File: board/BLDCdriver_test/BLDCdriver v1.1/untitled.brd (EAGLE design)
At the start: 46 x 65 mm, 28 parts, among them M1 JST-XH-03-PIN-LONG-PAD, X1 JST-XH-02-PIN-LONG-PAD, X2 JST-XH-06-PIN-ROUND-PAD, X4 JST-XH-04-PIN-ROUND-PAD

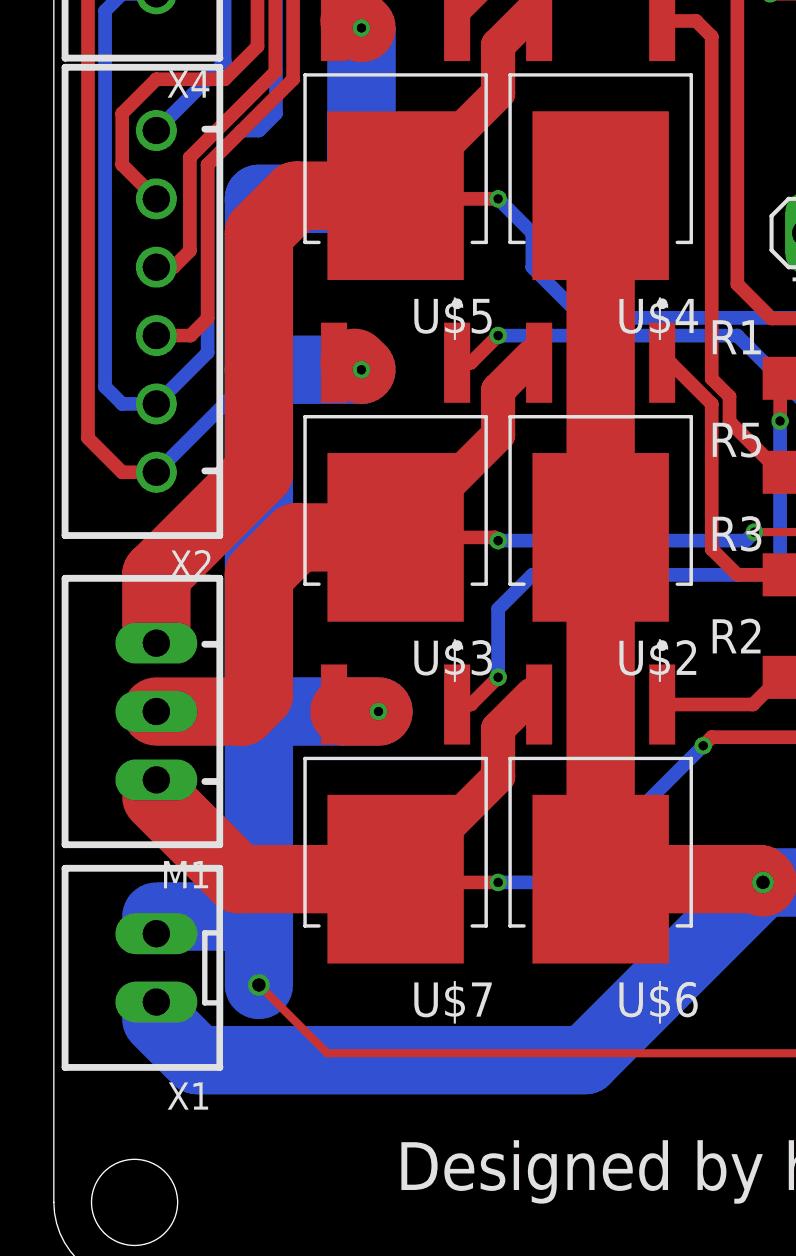
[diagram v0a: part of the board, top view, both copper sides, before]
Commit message: update motordriver
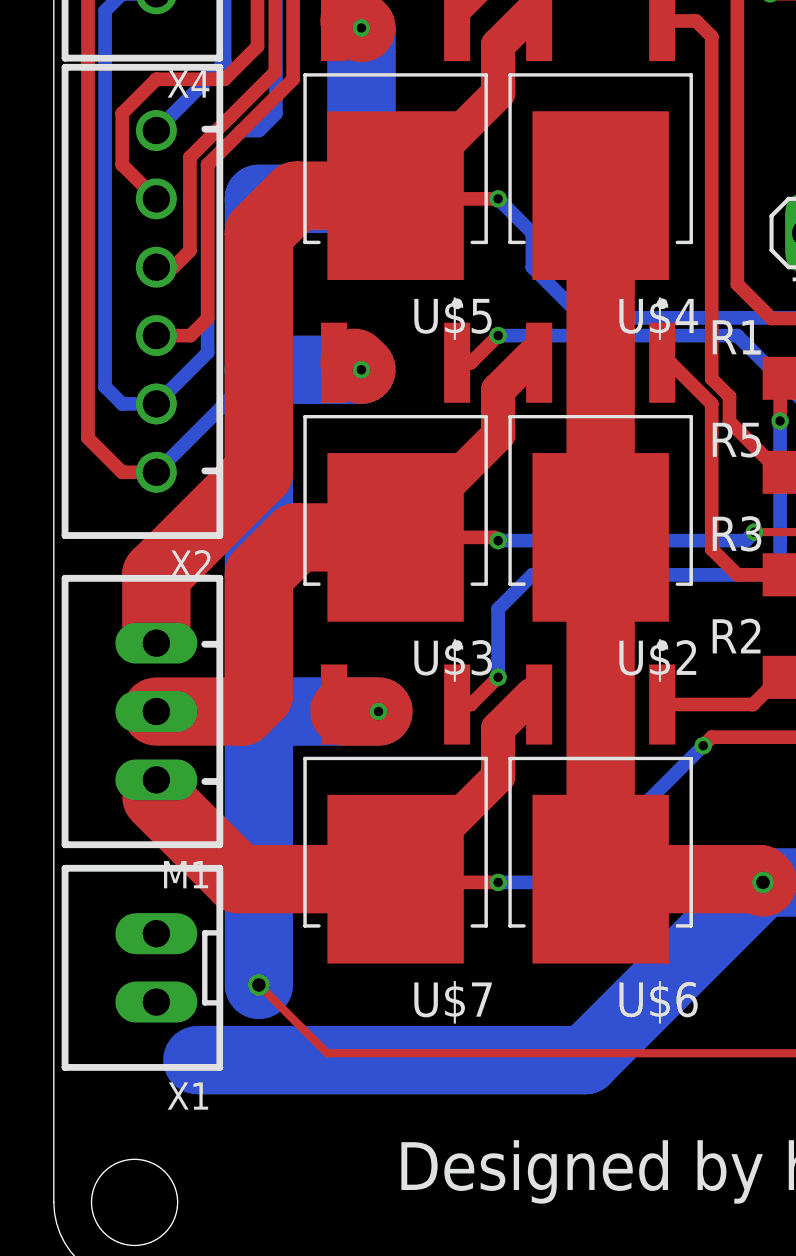
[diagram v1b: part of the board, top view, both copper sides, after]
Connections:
- net GND: now also X1.1; no longer X1.2
- net VCC: now also X1.2; no longer X1.1
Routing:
- net GND: track 201.4 -> 196.9 mm
- net VCC: track 89.3 -> 86.5 mm
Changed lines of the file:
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@@
 <contactref element="U$5" pad="3"/>
 <contactref element="U$1" pad="8"/>
-<contactref element="X1" pad="2"/>
 <via x="7.62" y="5.08" extent="1-16" drill="0.5"/>
-<wire x1="7.62" y1="5.08" x2="7.62" y2="7.62" width="2.54" layer="16"/>
-<wire x1="7.62" y1="7.62" x2="7.62" y2="15.24" width="2.54" layer="16"/>
+<wire x1="7.62" y1="5.08" x2="7.62" y2="15.24" width="2.54" layer="16"/>
 <wire x1="7.62" y1="15.24" x2="7.62" y2="27.94" width="2.54" layer="16"/>
 <contactref element="SV1" pad="2"/>
@@
 <wire x1="10.795" y1="34.29" x2="7.62" y2="34.29" width="2.54" layer="16"/>
 <wire x1="11.43" y1="40.64" x2="11.17" y2="40.9" width="2.54" layer="1"/>
-<wire x1="3.81" y1="6.985" x2="3.81" y2="7.62" width="0.3048" layer="16"/>
-<wire x1="3.81" y1="7.62" x2="7.62" y2="7.62" width="2.54" layer="16"/>
 <wire x1="10.535" y1="15.5" x2="10.795" y2="15.24" width="0.508" layer="1"/>
 <wire x1="10.795" y1="15.24" x2="12.065" y2="15.24" width="2.54" layer="1"/>
@@
 <wire x1="6.35" y1="39.37" x2="3.81" y2="36.83" width="0.508" layer="16"/>
 <wire x1="6.35" y1="44.45" x2="6.35" y2="39.37" width="0.508" layer="16"/>
+<contactref element="X1" pad="1"/>
+<wire x1="3.81" y1="4.445" x2="7.62" y2="5.08" width="0" layer="19" extent="1-1"/>
 </signal>
 <signal name="N$12">
@@
 <contactref element="D3" pad="A"/>
 <contactref element="U$1" pad="7"/>
-<contactref element="X1" pad="1"/>
 <wire x1="20.32" y1="9.01" x2="20.32" y2="21.71" width="2.54" layer="1"/>
-<wire x1="20.32" y1="22.86" x2="20.32" y2="34.41" width="2.54" layer="1"/>
+<wire x1="20.32" y1="21.71" x2="20.32" y2="34.41" width="2.54" layer="1"/>
 <wire x1="35.045" y1="12.7" x2="35.045" y2="8.89" width="1.27" layer="1"/>
 <wire x1="35.045" y1="8.89" x2="35.045" y2="5.08" width="1.27" layer="1"/>
@@
 <wire x1="39.7891" y1="22.225" x2="39.7891" y2="16.2941" width="0.3048" layer="1"/>
 <wire x1="39.7891" y1="16.2941" x2="36.195" y2="12.7" width="0.3048" layer="1"/>
-<wire x1="3.81" y1="4.445" x2="3.81" y2="3.81" width="0.508" layer="16"/>
-<wire x1="3.81" y1="3.81" x2="5.334" y2="2.286" width="2.54" layer="16"/>
 <wire x1="19.7485" y1="2.286" x2="26.3525" y2="8.89" width="2.54" layer="16"/>
 <wire x1="5.334" y1="2.286" x2="19.7485" y2="2.286" width="2.54" layer="16"/>
-<wire x1="20.32" y1="21.71" x2="20.32" y2="22.86" width="2.54" layer="1"/>
+<contactref element="X1" pad="2"/>
+<wire x1="5.334" y1="2.286" x2="3.81" y2="6.985" width="0" layer="19" extent="16-16"/>
 </signal>
 <signal name="N$15">

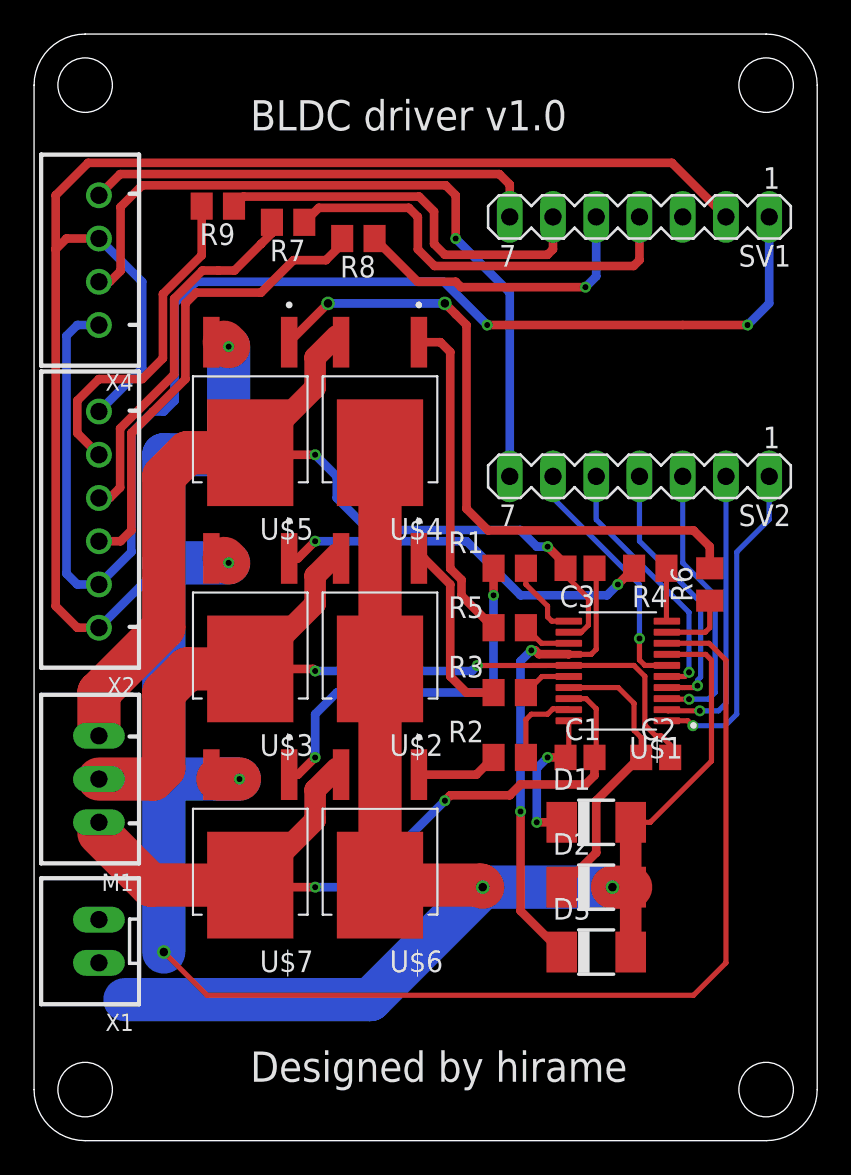
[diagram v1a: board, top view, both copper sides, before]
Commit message: marge前のファイル
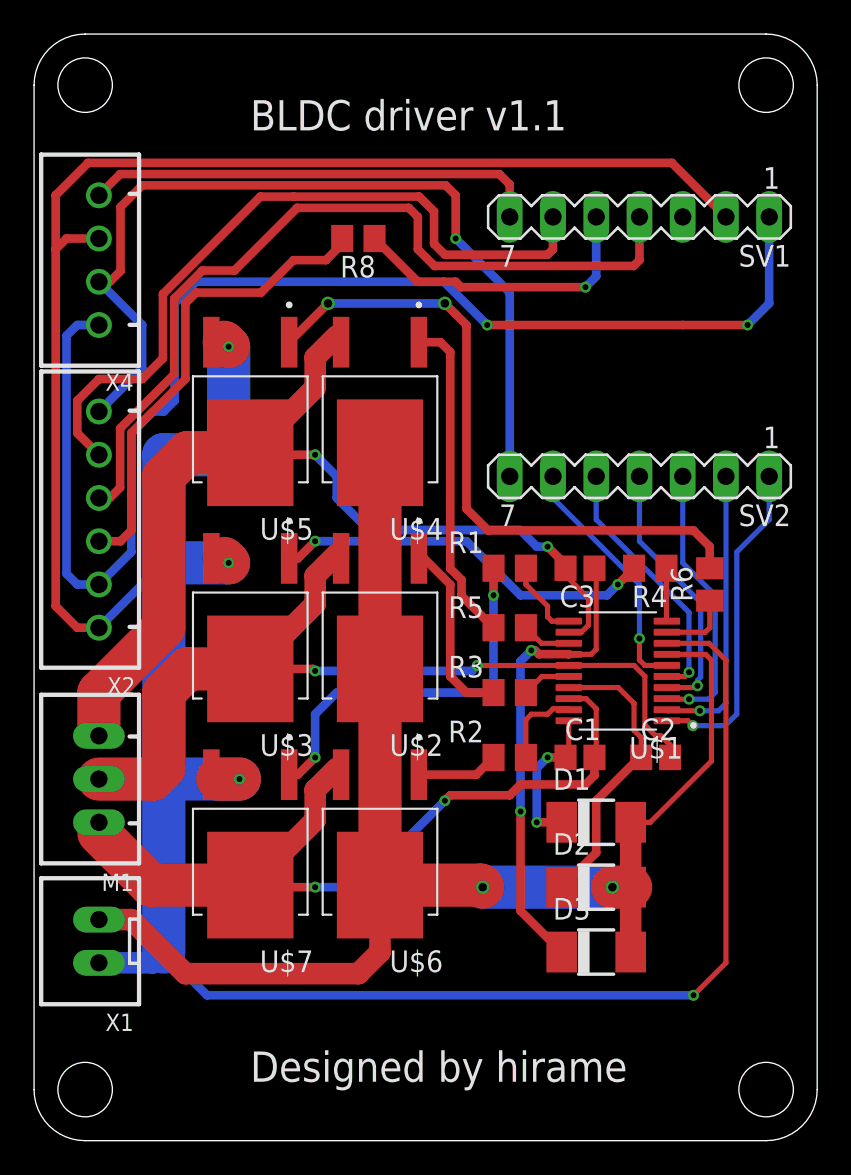
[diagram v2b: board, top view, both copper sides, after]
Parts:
- removed R7, R9: 300Ω, adafruit:M2012
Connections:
- removed net N$11: R7.1, SV1.4
- removed net N$20: R9.1, SV1.6
- net GND: no longer X2.6
- net MOSI: now also SV1.4; no longer R7.2
- net SCK: now also SV1.6; no longer R9.2
- net TX: now also X2.6
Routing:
- net MOSI: track 21.9 -> 48.7 mm
- net N$11: track 25.3 -> 0.00 mm
- net SCK: track 19.6 -> 43.4 mm
- net N$20: track 23.5 -> 0.00 mm
- net TX: track 43.6 -> 53.3 mm
- net GND: track 196.9 -> 188.7 mm
- net VCC: track 86.5 -> 85.0 mm
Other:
- board text added: "BLDC driver v1.1"
- board text removed: "BLDC driver v1.0"
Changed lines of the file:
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@@
 <?xml version="1.0" encoding="utf-8"?>
 <!DOCTYPE eagle SYSTEM "eagle.dtd">
-<eagle version="9.6.1">
+<eagle version="9.6.2">
 <drawing>
 <settings>
@@
 <wire x1="43" y1="-6" x2="46" y2="-3" width="0.001" layer="20" curve="90"/>
 <text x="12.7" y="-2.54" size="1.778" layer="25" font="vector">Designed by hirame</text>
-<text x="12.7" y="53.34" size="1.778" layer="25" font="vector">BLDC driver v1.0</text>
+<text x="12.7" y="53.34" size="1.778" layer="25" font="vector">BLDC driver v1.1</text>
 </plain>
 <attributes>
@@
 <attribute name="VALUE" x="-0.0825" y="39.7175" size="1.016" layer="27" ratio="10" rot="R90"/>
 </element>
-<element name="R7" library="adafruit" package="M2012" value="300Ω" x="14.9225" y="47.9425" smashed="yes" rot="R180">
-<attribute name="NAME" x="15.9385" y="46.9265" size="1.27" layer="25" rot="R180"/>
-<attribute name="VALUE" x="15.9385" y="50.2285" size="1.27" layer="27" rot="R180"/>
-</element>
 <element name="R8" library="adafruit" package="M2012" value="300Ω" x="19.05" y="46.99" smashed="yes" rot="R180">
 <attribute name="NAME" x="20.066" y="45.974" size="1.27" layer="25" rot="R180"/>
 <attribute name="VALUE" x="20.066" y="49.276" size="1.27" layer="27" rot="R180"/>
-</element>
-<element name="R9" library="adafruit" package="M2012" value="300Ω" x="10.795" y="48.895" smashed="yes" rot="R180">
-<attribute name="NAME" x="11.811" y="47.879" size="1.27" layer="25" rot="R180"/>
-<attribute name="VALUE" x="11.811" y="51.181" size="1.27" layer="27" rot="R180"/>
 </element>
 </elements>
@@
 <contactref element="U$5" pad="3"/>
 <contactref element="U$1" pad="8"/>
-<via x="7.62" y="5.08" extent="1-16" drill="0.5"/>
-<wire x1="7.62" y1="5.08" x2="7.62" y2="15.24" width="2.54" layer="16"/>
+<wire x1="7.62" y1="15.24" x2="7.62" y2="5.08" width="2.54" layer="16"/>
 <wire x1="7.62" y1="15.24" x2="7.62" y2="27.94" width="2.54" layer="16"/>
 <contactref element="SV1" pad="2"/>
@@
 <wire x1="39.65" y1="23.215" x2="40.64" y2="22.225" width="0.3048" layer="1"/>
 <wire x1="40.64" y1="22.225" x2="40.64" y2="4.445" width="0.3048" layer="1"/>
-<wire x1="38.735" y1="2.54" x2="10.16" y2="2.54" width="0.3048" layer="1"/>
-<wire x1="10.16" y1="2.54" x2="7.62" y2="5.08" width="0.3048" layer="1"/>
 <wire x1="11.17" y1="40.9" x2="10.414" y2="40.9" width="0.3048" layer="1"/>
 <via x="11.43" y="40.64" extent="1-16" drill="0.35"/>
@@
 <wire x1="7.62" y1="34.29" x2="7.62" y2="27.94" width="2.54" layer="16"/>
 <wire x1="10.414" y1="15.5" x2="10.535" y2="15.5" width="0.508" layer="1"/>
-<contactref element="X2" pad="6"/>
-<wire x1="3.81" y1="46.99" x2="6.35" y2="44.45" width="0.508" layer="16"/>
-<wire x1="6.35" y1="39.37" x2="3.81" y2="36.83" width="0.508" layer="16"/>
-<wire x1="6.35" y1="44.45" x2="6.35" y2="39.37" width="0.508" layer="16"/>
 <contactref element="X1" pad="1"/>
-<wire x1="3.81" y1="4.445" x2="7.62" y2="5.08" width="0" layer="19" extent="1-1"/>
+<wire x1="3.81" y1="4.445" x2="6.985" y2="4.445" width="1.27" layer="16"/>
+<wire x1="6.985" y1="4.445" x2="7.62" y2="5.08" width="1.27" layer="16"/>
+<wire x1="7.62" y1="5.08" x2="10.16" y2="2.54" width="0.508" layer="16"/>
+<wire x1="10.16" y1="2.54" x2="38.735" y2="2.54" width="0.508" layer="16"/>
+<via x="38.735" y="2.54" extent="1-16" drill="0.35"/>
 </signal>
 <signal name="N$12">
@@
 <wire x1="39.7891" y1="22.225" x2="39.7891" y2="16.2941" width="0.3048" layer="1"/>
 <wire x1="39.7891" y1="16.2941" x2="36.195" y2="12.7" width="0.3048" layer="1"/>
-<wire x1="19.7485" y1="2.286" x2="26.3525" y2="8.89" width="2.54" layer="16"/>
-<wire x1="5.334" y1="2.286" x2="19.7485" y2="2.286" width="2.54" layer="16"/>
 <contactref element="X1" pad="2"/>
-<wire x1="5.334" y1="2.286" x2="3.81" y2="6.985" width="0" layer="19" extent="16-16"/>
+<wire x1="3.81" y1="6.985" x2="5.715" y2="6.985" width="1.27" layer="1"/>
+<wire x1="8.89" y1="3.81" x2="19.05" y2="3.81" width="1.27" layer="1"/>
+<wire x1="19.05" y1="3.81" x2="20.32" y2="5.08" width="1.27" layer="1"/>
+<wire x1="20.32" y1="5.08" x2="20.32" y2="9.01" width="1.27" layer="1"/>
+<wire x1="5.715" y1="6.985" x2="8.89" y2="3.81" width="1.27" layer="1"/>
 </signal>
 <signal name="N$15">
@@
 <wire x1="5.0546" y1="35.83355" x2="8.2296" y2="39.00855" width="0.508" layer="1"/>
 <wire x1="8.2296" y1="39.00855" x2="8.2296" y2="43.45355" width="0.508" layer="1"/>
-<contactref element="R7" pad="2"/>
-<wire x1="13.9725" y1="47.31" x2="13.9725" y2="47.9425" width="0.508" layer="1"/>
-<wire x1="9.88645" y1="45.1104" x2="10.8204" y2="45.1104" width="0.508" layer="1"/>
-<wire x1="13.335" y1="46.6725" x2="13.9725" y2="47.31" width="0.508" layer="1"/>
-<wire x1="10.8204" y1="45.1104" x2="11.7729" y2="45.1104" width="0.508" layer="1"/>
-<wire x1="11.7729" y1="45.1104" x2="13.335" y2="46.6725" width="0.508" layer="1"/>
+<wire x1="9.88645" y1="45.1104" x2="11.7729" y2="45.1104" width="0.508" layer="1"/>
+<contactref element="SV1" pad="4"/>
+<wire x1="22.0091" y1="48.7934" x2="22.5425" y2="48.26" width="0.508" layer="1"/>
+<wire x1="35.2171" y1="45.3771" x2="35.56" y2="45.72" width="0.508" layer="1"/>
+<wire x1="35.56" y1="45.72" x2="35.56" y2="48.26" width="0.508" layer="1"/>
+<wire x1="22.5425" y1="48.26" x2="22.5425" y2="46.355" width="0.508" layer="1"/>
+<wire x1="22.5425" y1="46.355" x2="23.5204" y2="45.3771" width="0.508" layer="1"/>
+<wire x1="23.5204" y1="45.3771" x2="35.2171" y2="45.3771" width="0.508" layer="1"/>
+<wire x1="15.4559" y1="48.7934" x2="22.0091" y2="48.7934" width="0.508" layer="1"/>
+<wire x1="11.7729" y1="45.1104" x2="15.4559" y2="48.7934" width="0.508" layer="1"/>
 </signal>
 <signal name="SCK">
@@
 <wire x1="2.54" y1="37.465" x2="3.81" y2="38.735" width="0.508" layer="1"/>
 <wire x1="7.5692" y1="39.9542" x2="7.5692" y2="43.7271" width="0.508" layer="1"/>
-<contactref element="R9" pad="2"/>
-<wire x1="9.845" y1="46.0029" x2="9.845" y2="48.895" width="0.508" layer="1"/>
-<wire x1="7.5692" y1="43.7271" x2="9.845" y2="46.0029" width="0.508" layer="1"/>
+<contactref element="SV1" pad="6"/>
+<wire x1="22.6187" y1="49.4538" x2="23.495" y2="48.5775" width="0.508" layer="1"/>
+<wire x1="23.495" y1="46.6725" x2="24.13" y2="46.0375" width="0.508" layer="1"/>
+<wire x1="30.1625" y1="46.0375" x2="30.48" y2="46.355" width="0.508" layer="1"/>
+<wire x1="30.48" y1="46.355" x2="30.48" y2="48.26" width="0.508" layer="1"/>
+<wire x1="15.24" y1="49.4538" x2="22.6187" y2="49.4538" width="0.508" layer="1"/>
+<wire x1="23.495" y1="48.5775" x2="23.495" y2="46.6725" width="0.508" layer="1"/>
+<wire x1="24.13" y1="46.0375" x2="30.1625" y2="46.0375" width="0.508" layer="1"/>
+<wire x1="13.2959" y1="49.4538" x2="15.24" y2="49.4538" width="0.508" layer="1"/>
+<wire x1="7.5692" y1="43.7271" x2="13.2959" y2="49.4538" width="0.508" layer="1"/>
 </signal>
 <signal name="RX">
@@
 <wire x1="5.08" y1="45.085" x2="5.08" y2="48.8442" width="0.508" layer="1"/>
 <wire x1="6.35" y1="50.1142" x2="24.1808" y2="50.1142" width="0.508" layer="1"/>
+<contactref element="X2" pad="6"/>
+<wire x1="6.35" y1="39.37" x2="6.35" y2="41.91" width="0.508" layer="16"/>
+<wire x1="6.35" y1="41.91" x2="3.81" y2="44.45" width="0.508" layer="16"/>
+<wire x1="3.81" y1="36.83" x2="6.35" y2="39.37" width="0.508" layer="16"/>
 </signal>
 <signal name="LC">
@@
 <wire x1="41.275" y1="19.05" x2="41.275" y2="28.575" width="0.3048" layer="16"/>
 </signal>
-<signal name="N$11">
-<contactref element="SV1" pad="4"/>
-<contactref element="R7" pad="1"/>
-<wire x1="15.8725" y1="47.9425" x2="16.7234" y2="48.7934" width="0.508" layer="1"/>
-<wire x1="22.0091" y1="48.7934" x2="22.5425" y2="48.26" width="0.508" layer="1"/>
-<wire x1="35.2171" y1="45.3771" x2="35.56" y2="45.72" width="0.508" layer="1"/>
-<wire x1="35.56" y1="45.72" x2="35.56" y2="48.26" width="0.508" layer="1"/>
-<wire x1="16.7234" y1="48.7934" x2="22.0091" y2="48.7934" width="0.508" layer="1"/>
-<wire x1="22.5425" y1="48.26" x2="22.5425" y2="46.355" width="0.508" layer="1"/>
-<wire x1="22.5425" y1="46.355" x2="23.5204" y2="45.3771" width="0.508" layer="1"/>
-<wire x1="23.5204" y1="45.3771" x2="35.2171" y2="45.3771" width="0.508" layer="1"/>
-</signal>
-<signal name="N$20">
-<contactref element="SV1" pad="6"/>
-<contactref element="R9" pad="1"/>
-<wire x1="11.745" y1="48.895" x2="12.3038" y2="49.4538" width="0.508" layer="1"/>
-<wire x1="22.6187" y1="49.4538" x2="23.495" y2="48.5775" width="0.508" layer="1"/>
-<wire x1="23.495" y1="46.6725" x2="24.13" y2="46.0375" width="0.508" layer="1"/>
-<wire x1="30.1625" y1="46.0375" x2="30.48" y2="46.355" width="0.508" layer="1"/>
-<wire x1="30.48" y1="46.355" x2="30.48" y2="48.26" width="0.508" layer="1"/>
-<wire x1="12.3038" y1="49.4538" x2="22.6187" y2="49.4538" width="0.508" layer="1"/>
-<wire x1="23.495" y1="48.5775" x2="23.495" y2="46.6725" width="0.508" layer="1"/>
-<wire x1="24.13" y1="46.0375" x2="30.1625" y2="46.0375" width="0.508" layer="1"/>
-</signal>
 <signal name="N$21">
